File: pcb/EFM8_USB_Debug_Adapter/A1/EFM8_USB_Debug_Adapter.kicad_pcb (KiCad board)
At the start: 2 copper layers, 55 x 45 mm, 35 parts, among them J100 EFM8_IDC_Debug_Header_Horizon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, J110 2137160001, J111 TTL-232R_Header_Horizontal, J120 31230102, J130 EFM8_USB_8-Bit_Debug_Header_H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, M101 DBG8_Light_Pipe, M102 USB_Light_Pipe, Q110 SI3443CDV-T1-GE3, Q111 DMMT5401, Q120 SI3443CDV-T1-GE3, Q121 DMMT5401, Q130 SI3443CDV-T1-GE3, Q131 DMMT5401

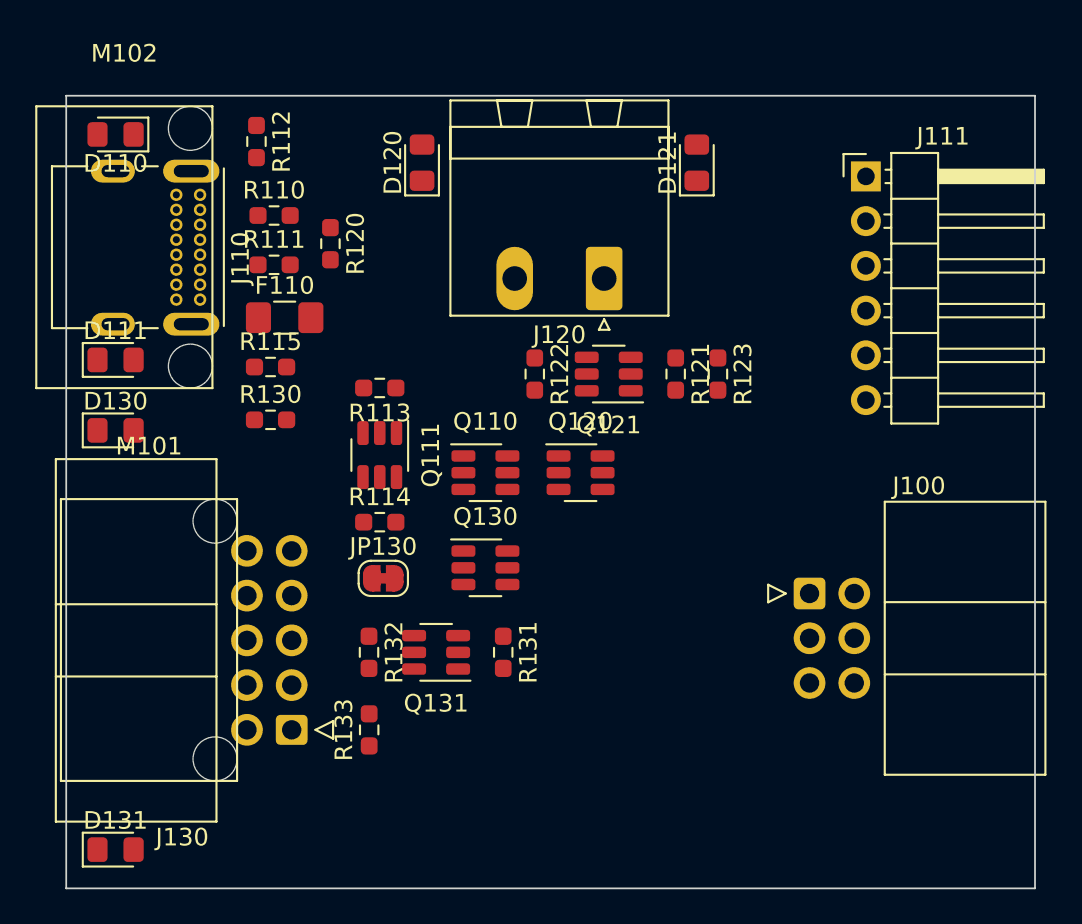
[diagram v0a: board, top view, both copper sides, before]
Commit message: Lightpipes aktualisiert
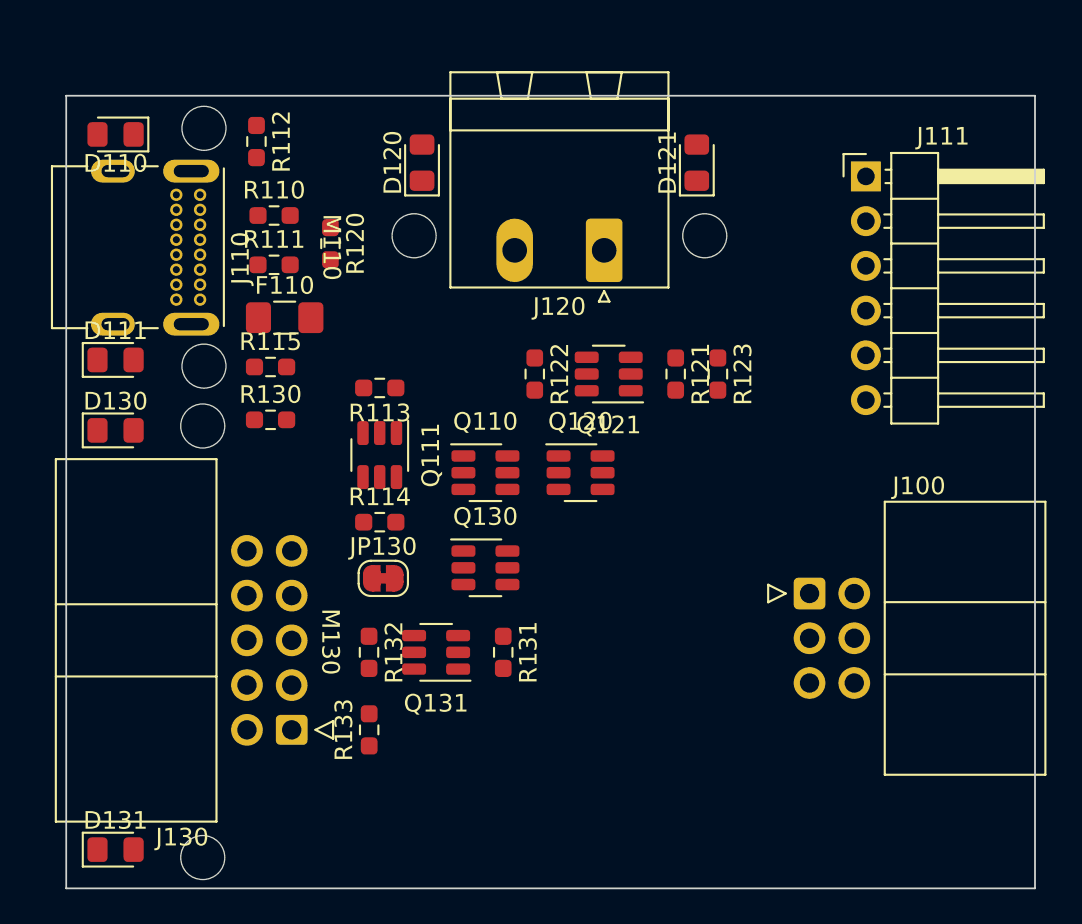
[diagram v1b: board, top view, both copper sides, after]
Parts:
- added M120: PSU_Light_Pipe, Mechanical_User:PSU_CON_Light_Pipe, F.Cu at (124.0, 35.5)
- moved J120 1.60 mm to (126.5, 39.8)
- moved M110 0.77 mm to (100.1, 39.6), turned to -90 degrees
- moved M130 0.71 mm to (100.0, 62.0), turned to -90 degrees
- renumbered M102 to M110, M101 to M130
